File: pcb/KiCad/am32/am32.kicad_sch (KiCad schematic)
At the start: 63 parts, among them IC1 STM32G071CBU6, Q1 TPHR8504PL_L1Q, Q2 TPHR8504PL_L1Q, Q3 TPHR8504PL_L1Q, Q4 TPHR8504PL_L1Q, Q5 TPHR8504PL_L1Q, Q6 TPHR8504PL_L1Q, U1 TS3480CX33 RFG, U4 INA180B3IDBVR

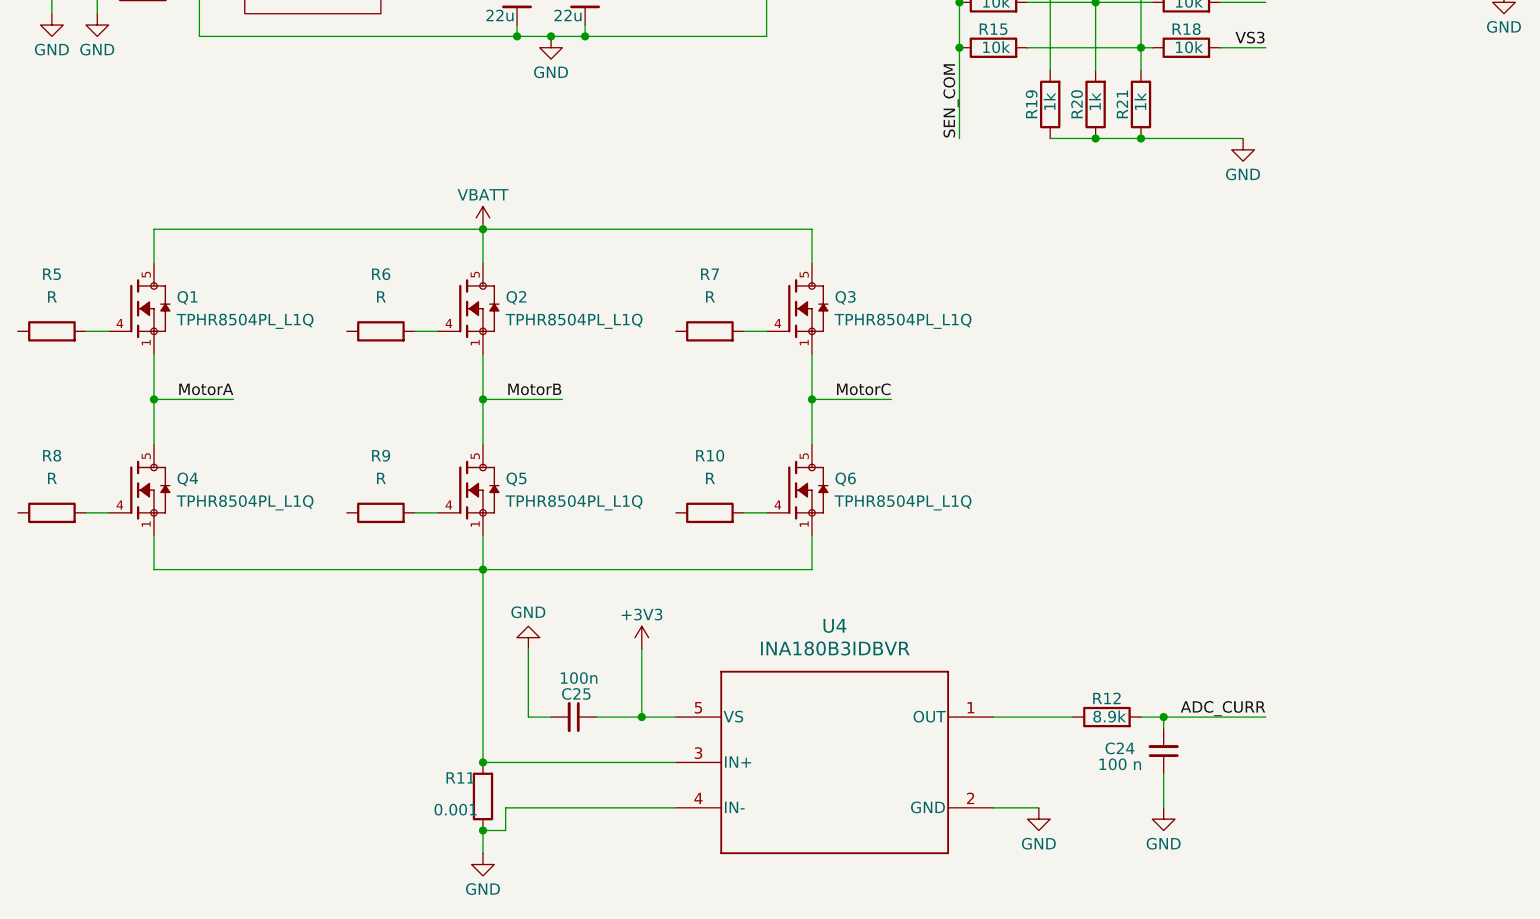
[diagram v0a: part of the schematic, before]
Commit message: Adding leftovers
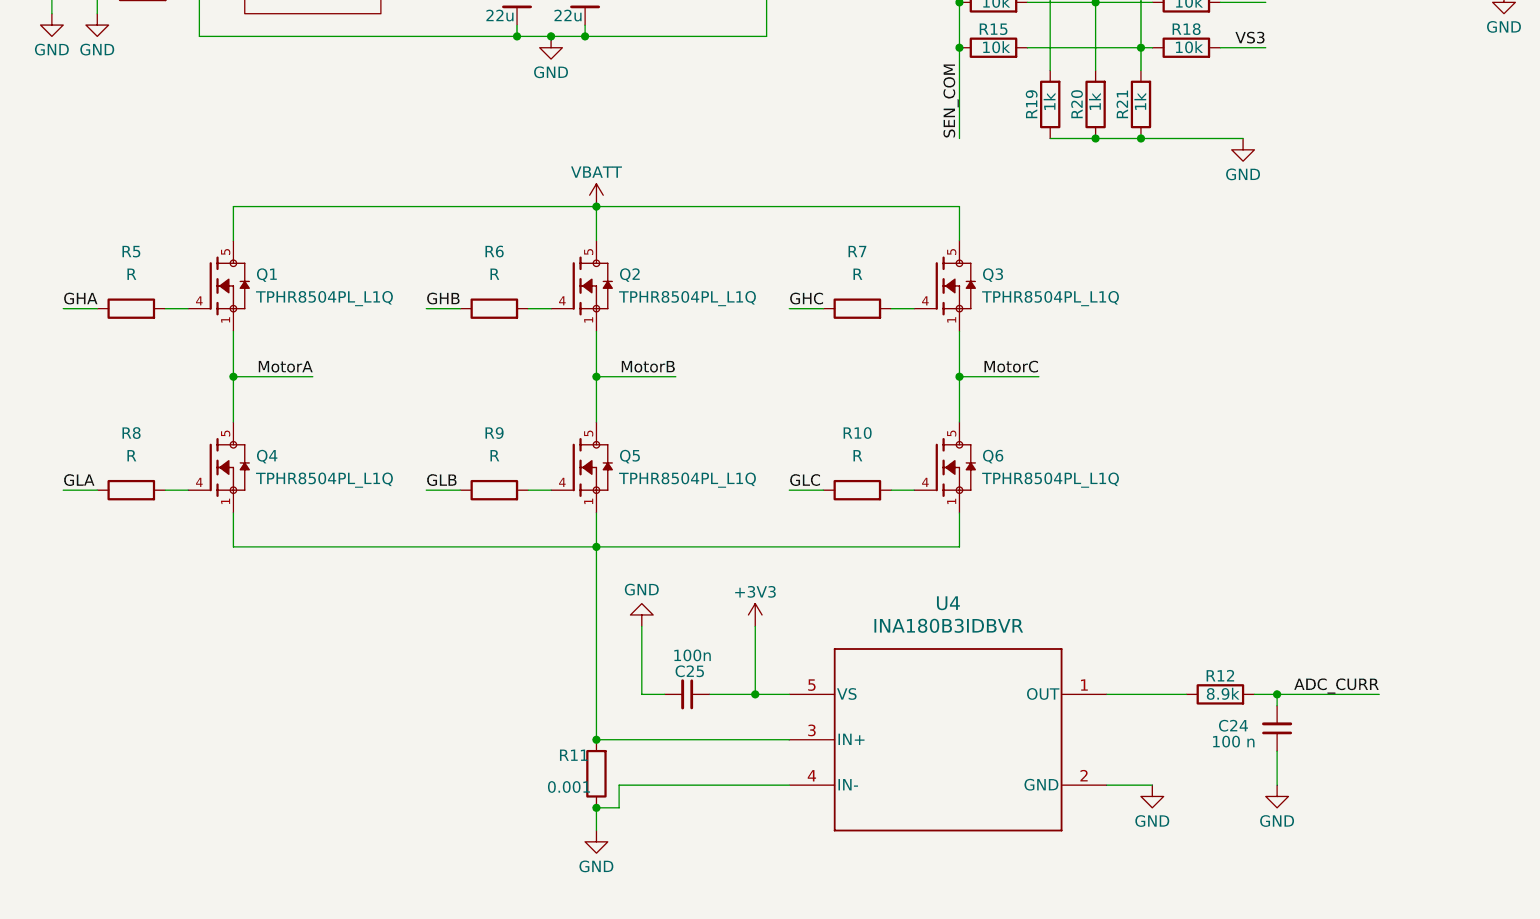
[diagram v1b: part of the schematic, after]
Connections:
- net GHA: now also R5.1
- net GHB: now also R6.1
- net GHC: now also R7.1
- net GLA: now also R8.1
- net GLB: now also R9.1
- net GLC: now also R10.1
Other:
- moved on the sheet: C24, C25, Q1, Q2, Q3, Q4, Q5, Q6, R10, R11, R12, R5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
